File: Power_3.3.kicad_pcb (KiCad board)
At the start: 2 copper layers, 68 x 60 mm, 12 parts, among them J1 Conn_01x03, J2 Conn_01x02

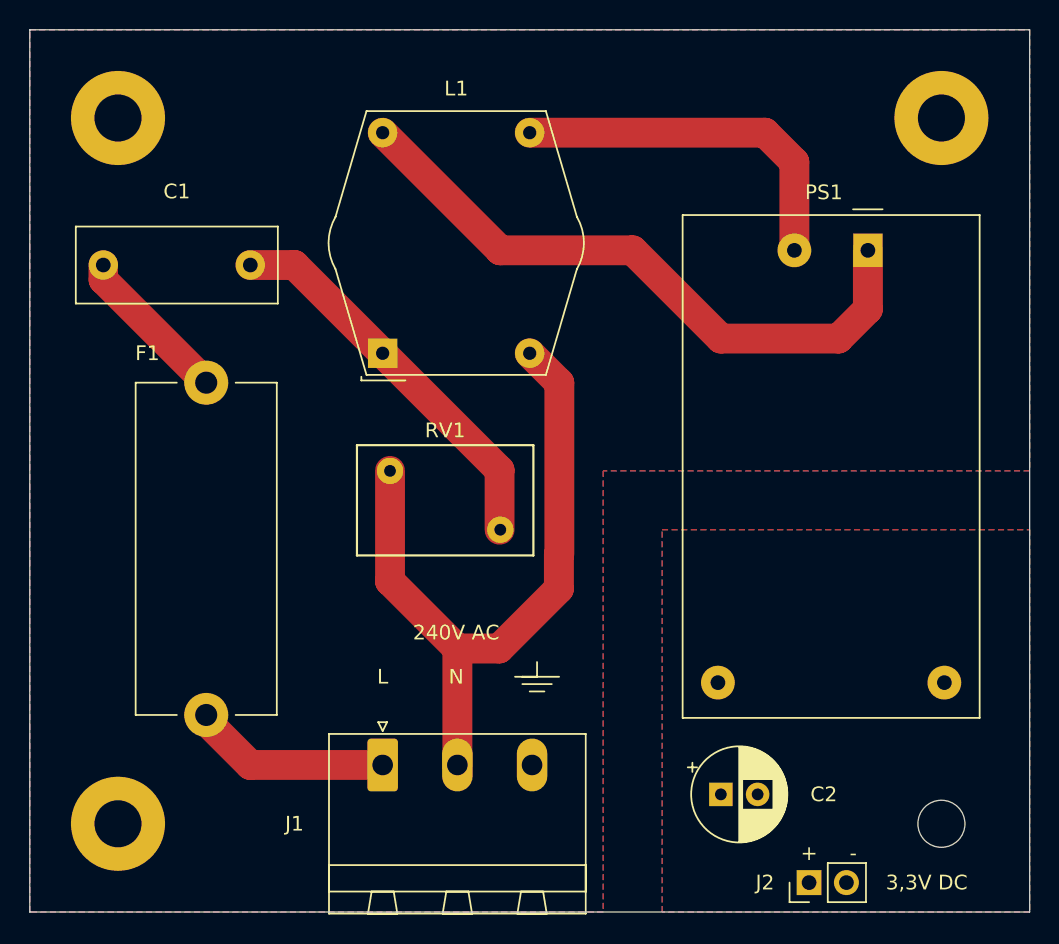
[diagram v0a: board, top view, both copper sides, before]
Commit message: neue Plazireung der Bauteile
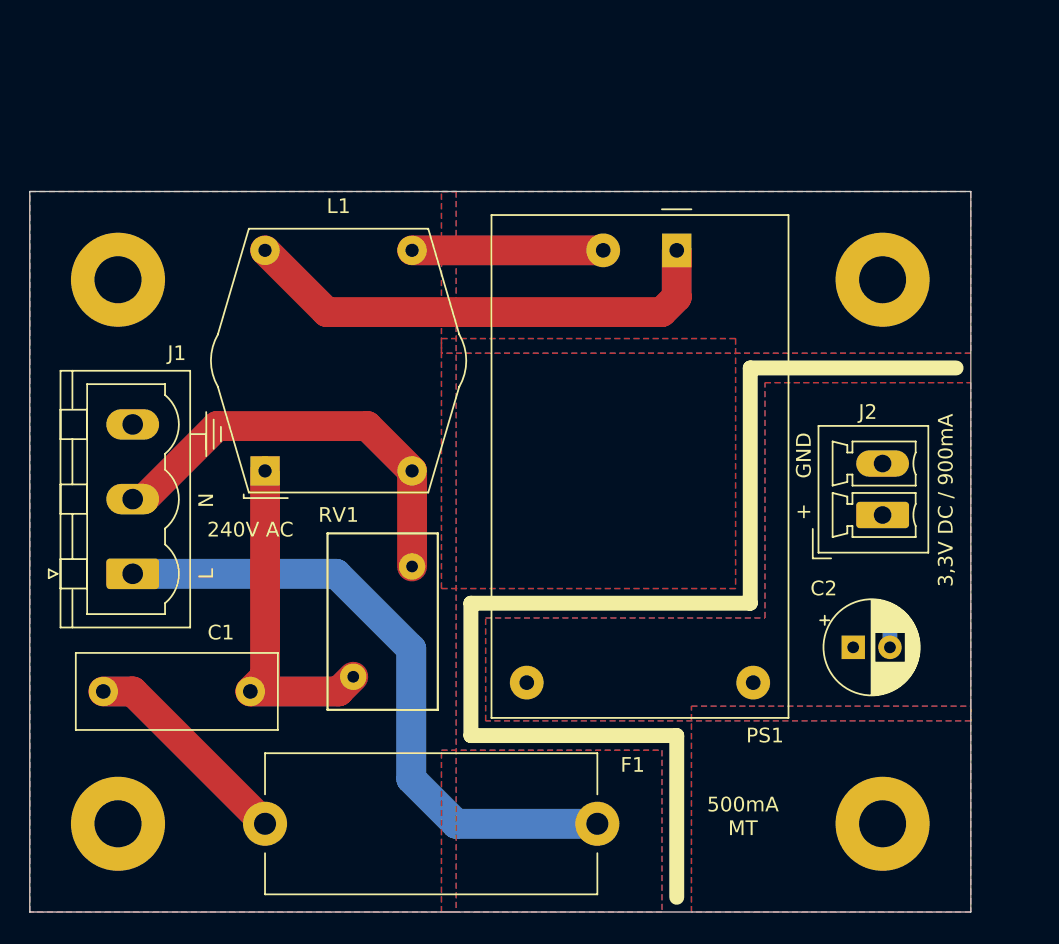
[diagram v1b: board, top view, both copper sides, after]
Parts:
- H1: value MountingHole -> MountingHole_Pad; footprint MountingHole:MountingHole_3.2mm_M3 -> MountingHole:MountingHole_3.2mm_M3_Pad
- J1: footprint Connector_Phoenix_MSTB:PhoenixContact_MSTBA_2,5_3-G-5,08_1x03_P5.08mm_Horizontal -> Connector_Phoenix_MSTB:PhoenixContact_MSTBVA_2,5_3-G-5,08_1x03_P5.08mm_Vertical
- J2: footprint Connector_PinHeader_2.54mm:PinHeader_1x02_P2.54mm_Vertical -> Connector_Phoenix_MC:PhoenixContact_MCV_1,5_2-G-3.5_1x02_P3.50mm_Vertical
- moved F1 30.3 mm to (76.0, 114.0), turned to 0 degrees
- moved C1 29.0 mm to (75.0, 105.0)
- moved J2 25.5 mm to (118.0, 93.0)
- moved J1 21.4 mm to (67.0, 97.0), turned to 90 degrees
- moved RV1 14.1 mm to (82.0, 104.0), turned to 90 degrees
- moved C2 13.5 mm to (116.0, 102.0)
- moved PS1 13.0 mm to (104.0, 75.0)
- moved H2 11.7 mm to (118.0, 77.0)
- moved L1 11.3 mm to (76.0, 90.0)
- moved H3 11.0 mm to (66.0, 77.0)
- moved H1 4.00 mm to (118.0, 114.0)
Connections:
- net Net-(F1-Pad2) renamed /L
- net Net-(J1-Pad2) renamed /N
- H1 pad 1: (no net) -> /GND
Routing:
- net /L: track 13.6 -> 44.6 mm
- net /N: track 47.3 -> 28.8 mm
- net Net-(L1-Pad4): track 24.8 -> 13.0 mm
- net Net-(L1-Pad2): track 43.6 -> 33.3 mm
- net Net-(C1-Pad1): track 26.8 -> 22.8 mm
- net Net-(C1-Pad2): track 10.9 -> 14.7 mm
- net /GND: track 0.00 -> 1.19 mm
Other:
- board size 68 x 60 mm -> 64 x 49 mm
- net class 240V: clearance 2.032 -> 1.016
- board text added: "3,3V DC / 900mA"
- board text added: "500mA MT"
- board text added: "GND"
- board text added: "Power 3W In : 240V AC Out : 3.3V DC / 900mA PSch 11/21 - V1.0"
- board text removed: "-"
- board text removed: "3,3V DC"
- board text removed: "Power 3W In : 240V AC Out : 3.3V DC PSch 11/21 - V1.0"
